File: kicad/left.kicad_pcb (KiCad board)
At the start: 4 copper layers, 127.3 x 89.6 mm, 158 parts, among them M2 MountingHole_2.2mm_M2, Q1 PMF170XP,115, Q2 FS8205A_C2830320, SW1 TS-1088-AR02016, U1 TLV7031QDCKRQ1, U2 E73-2G4M08S1C, U3 SN74LVC1G74DQER, U4 S2B-PH-K-S(LF)(SN), U5 BL8573CS8TR, U6 DW01A_C42380662, U7 LP5024RSMR, X1 FC-13532.768KHZ9PF20PPM

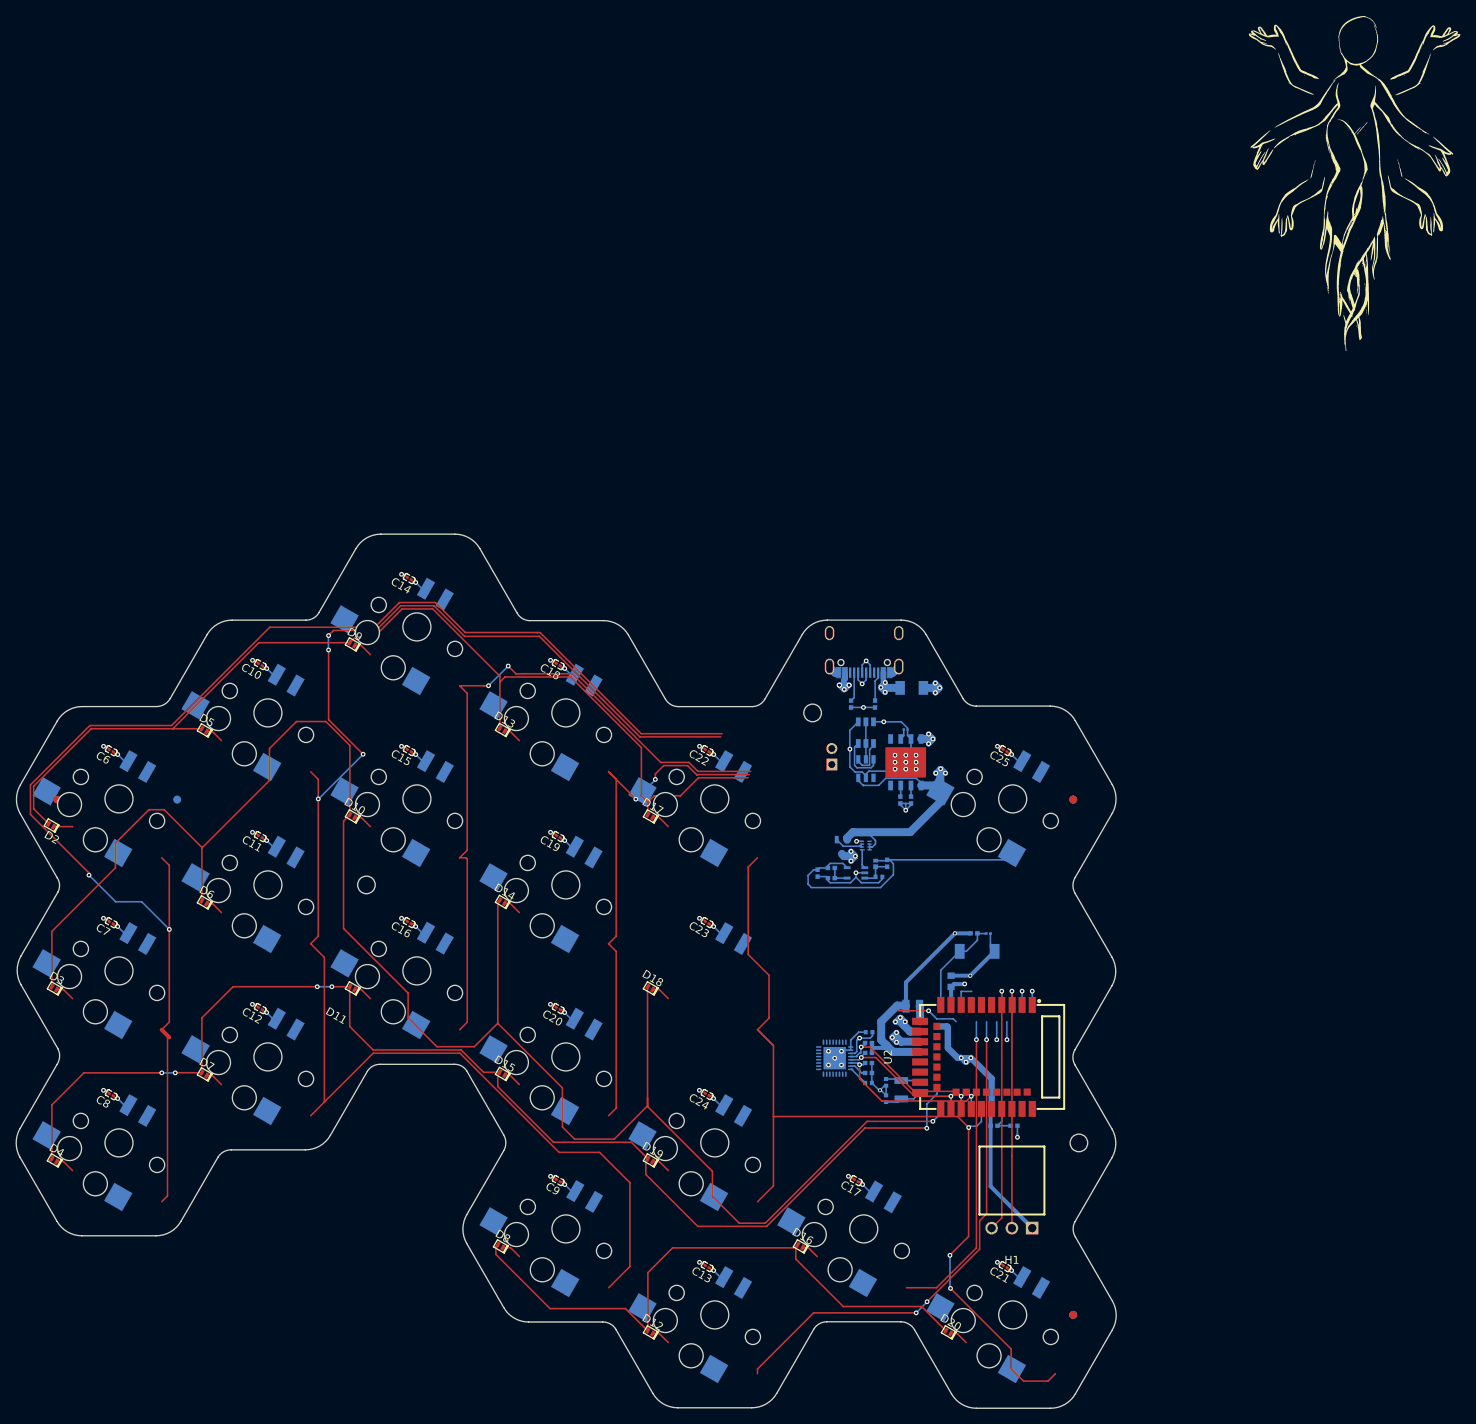
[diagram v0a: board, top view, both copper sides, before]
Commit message: ...
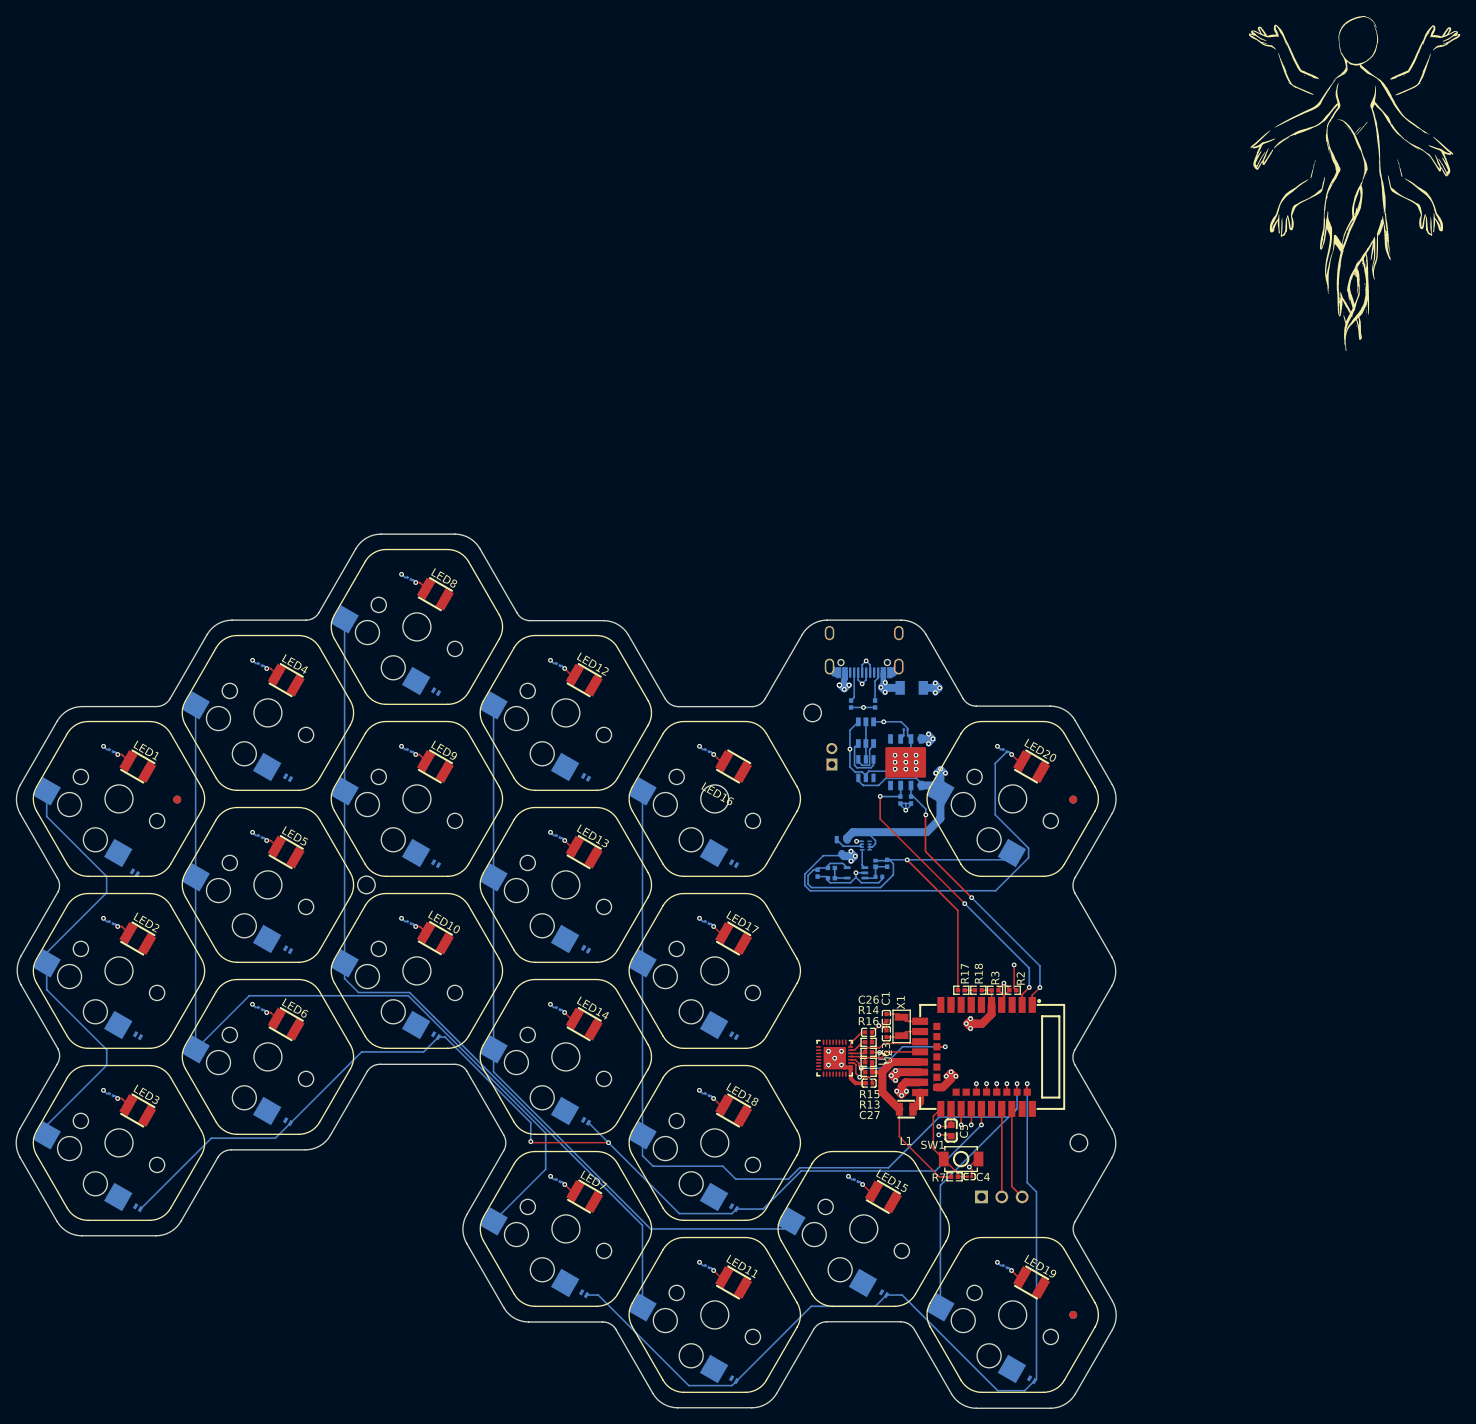
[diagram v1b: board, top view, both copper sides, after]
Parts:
- added R17: RC0402FR-071ML, easyeda2kicad:R0402, F.Cu at (138.2, 72.8)
- added R18: WR04W2494FTL, easyeda2kicad:R0402, F.Cu at (140.3, 72.8)
- added S17: Choc HEX, hexcaps:PG1350_hotswap_reversed, F.Cu at (107.4, 70.4)
- C1, C26, C27, C3, C4, C5, L1, LED1, LED10, LED11, LED12, LED13, LED14, LED15, LED16, LED17, LED18, LED19, LED2, LED20, LED3, LED4, LED5, LED6, LED7, LED8, LED9, R13, R14, R15, R16, R2, R3, R7, SW1, U7, X1: moved to F.Cu
- C10, C11, C12, C13, C14, C15, C16, C17, C18, C19, C20, C21, C22, C23, C24, C25, C6, C7, C8, C9, D10, D11, D12, D13, D14, D15, D16, D17, D18, D19, D2, D20, D3, D4, D5, D6, D7, D8, D9, H1: moved to B.Cu
- moved R7 30.5 mm to (137.3, 96.2)
- moved C4 30.5 mm to (139.2, 96.1)
- moved SW1 26.0 mm to (138.1, 93.9)
- moved C5 18.6 mm to (136.9, 90.4), turned to -90 degrees
- moved R2 16.9 mm to (144.6, 72.8)
- moved R3 16.9 mm to (142.4, 72.8)
- moved Fi2 15.0 mm to (40.2, 49.0)
- moved L1 12.9 mm to (131.3, 87.7)
- moved D8 12.0 mm to (91.0, 110.8), turned to -30 degrees
- moved D10 12.0 mm to (72.5, 57.0), turned to -30 degrees
- moved D5 12.0 mm to (54.0, 46.3), turned to -30 degrees
- moved D9 12.0 mm to (72.5, 35.5), turned to -30 degrees
- moved D11 12.0 mm to (72.5, 78.5), turned to -30 degrees
- moved D2 12.0 mm to (34.9, 58.2), turned to -30 degrees
- moved D3 12.0 mm to (35.3, 78.5), turned to -30 degrees
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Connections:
- U2 pad 1: /COL7 -> /STDBY
- U2 pad 12: /ROW3 -> unconnected-(U2-P0.26-Pad12)
- U2 pad 15: unconnected-(U2-AI3-Pad15) -> /LED_EN
- U2 pad 16: unconnected-(U2-P0.08-Pad16) -> /LED_SDA
- U2 pad 17: /COL6 -> /LED_SCL
- U2 pad 2: unconnected-(U2-P1.10-Pad2) -> /CHRG
- U2 pad 28: /ROW1 -> unconnected-(U2-P15-Pad28)
- U2 pad 3: unconnected-(U2-P0.03-Pad3) -> /PWR_BTN_PRESS
- U2 pad 32: /COL4 -> /COL1
- U2 pad 33: unconnected-(U2-P0.13-Pad33) -> /ROW3
- U2 pad 34: /COL3 -> /COL2
- U2 pad 36: /COL2 -> /COL3
- U2 pad 37: /SWDIO -> /SWBCLK
- U2 pad 38: /COL1 -> /COL4
- U2 pad 39: /SWBCLK -> /SWDIO
- U2 pad 40: unconnected-(U2-P1.04-Pad40) -> /COL5
- U2 pad 41: /STDBY -> unconnected-(U2-NF1-Pad41)
- U2 pad 42: unconnected-(U2-P1.06-Pad42) -> /ROW4
- U2 pad 43: /CHRG -> unconnected-(U2-NF2-Pad43)
- U2 pad 6: /COL5 -> unconnected-(U2-P1.13-Pad6)
- U2 pad 7: /LED_EN -> unconnected-(U2-AI0-Pad7)
- U2 pad 8: /LED_SDA -> unconnected-(U2-AI5-Pad8)
- U2 pad 9: /LED_SCL -> /ROW1
- U7 pad 1: /LED19 -> /LED20
- U7 pad 10: /LED3 -> /LED17
- U7 pad 11: /LED2 -> /LED13
- U7 pad 12: /LED5 -> /LED9
- U7 pad 13: /LED9 -> /LED5
- U7 pad 14: /LED13 -> /LED2
- U7 pad 15: /LED17 -> /LED3
- U7 pad 17: /LED1 -> /LED6
- U7 pad 18: /LED4 -> /LED10
- U7 pad 19: /LED8 -> /LED14
- U7 pad 2: /LED15 -> unconnected-(U7-OUT1-Pad2)
- U7 pad 20: /LED12 -> /LED18
- U7 pad 21: /LED16 -> /LED7
- U7 pad 22: unconnected-(U7-OUT21-Pad22) -> /LED11
- U7 pad 23: unconnected-(U7-OUT22-Pad23) -> /LED15
- U7 pad 24: /LED20 -> /LED19
- U7 pad 3: /LED11 -> unconnected-(U7-OUT2-Pad3)
- U7 pad 4: /LED7 -> /LED16
- U7 pad 5: /LED18 -> /LED12
- U7 pad 6: /LED14 -> /LED8
- U7 pad 7: /LED10 -> /LED4
- U7 pad 8: /LED6 -> /LED1
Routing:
- net /COL3: track 342.4 -> 106.2 mm, vias 10 -> 1
- net /ROW2: track 234.1 -> 0.00 mm, vias 1 -> 0
- net /ROW3: track 334.0 -> 134.7 mm, vias 8 -> 3
- net /ROW1: track 138.5 -> 0.00 mm, vias 1 -> 0
- net /COL2: track 0.00 -> 111.3 mm, vias 0 -> 1
- net /CHRG: track 122.2 -> 38.1 mm, vias 4 -> 3
- net /COL5: track 66.3 -> 130.1 mm, vias 2 -> 1
- net /COL1: track 0.00 -> 56.4 mm, vias 0 -> 1
- net /PWR: track 63.6 -> 119.5 mm
- net /COL4: track 39.1 -> 92.6 mm
- net /ROW4: track 76.2 -> 109.7 mm, vias 0 -> 1
- net /STDBY: track 3.11 -> 34.7 mm, vias 1 -> 3
- net GND: track 118.2 -> 96.7 mm, vias 47 -> 52
- net /SWDIO: track 31.9 -> 11.5 mm, vias 1 -> 0
- net /SWBCLK: track 31.3 -> 11.3 mm, vias 1 -> 0
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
